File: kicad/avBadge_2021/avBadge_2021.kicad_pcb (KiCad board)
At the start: 2 copper layers, 115 x 75 mm, 37 parts, among them J1 AVR-ISP-6, Q1 2N3904, SW1 SW_Push_Dual, SW2 SW_SPDT, U1 ATtiny84A-SSU

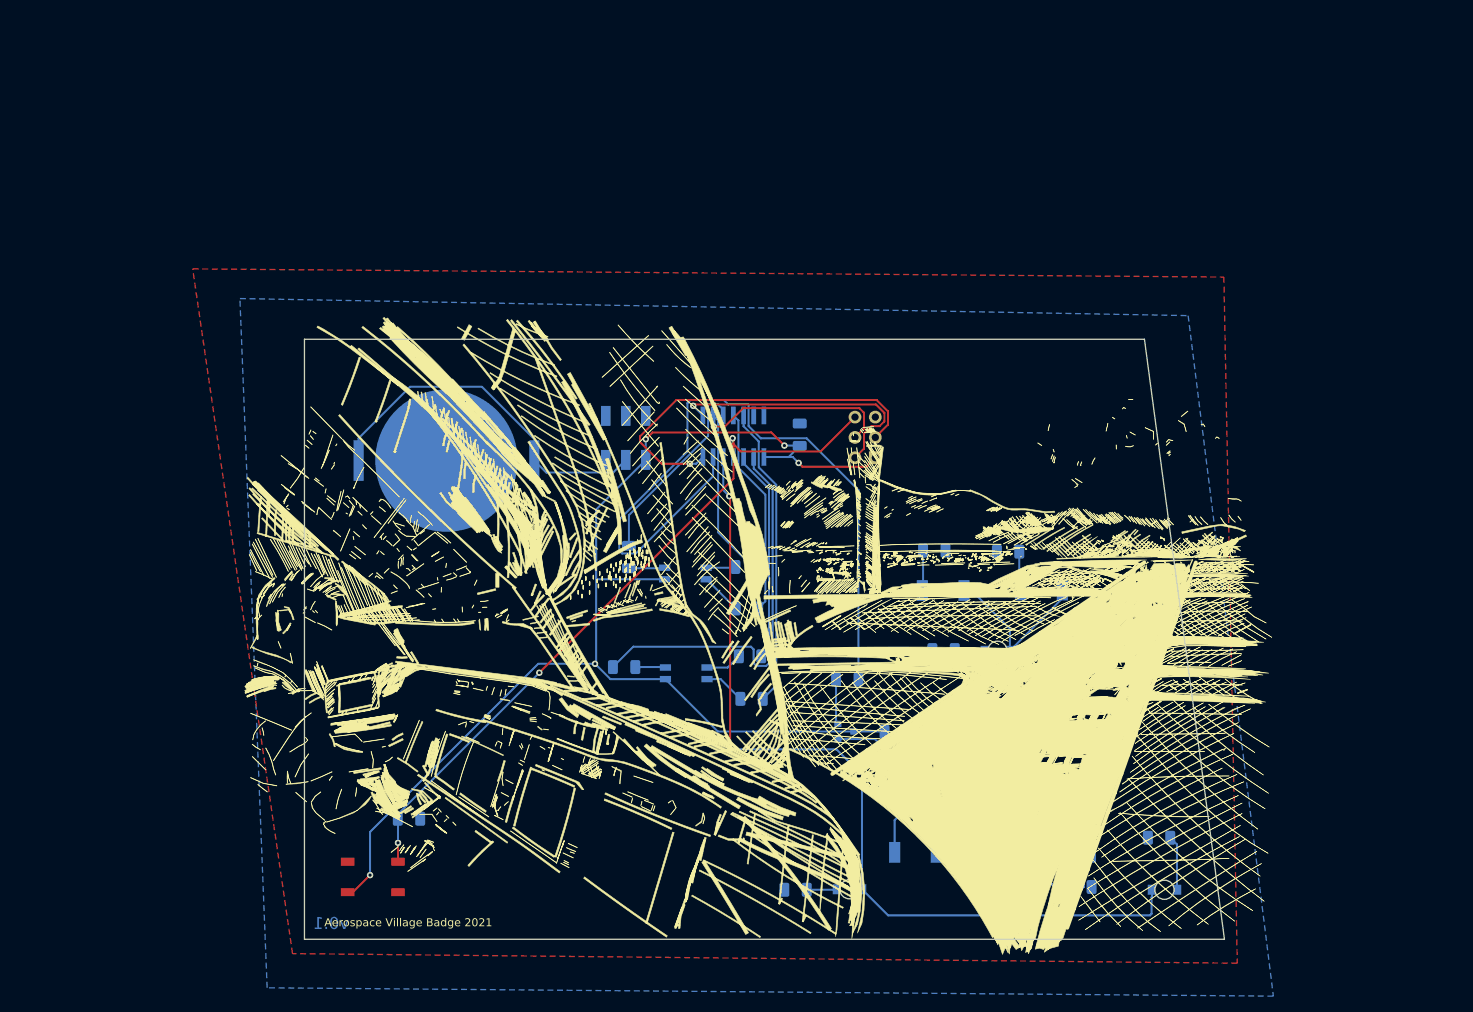
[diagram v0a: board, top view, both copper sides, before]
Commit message: v0.2 gerber builtout and sent for fabrication.
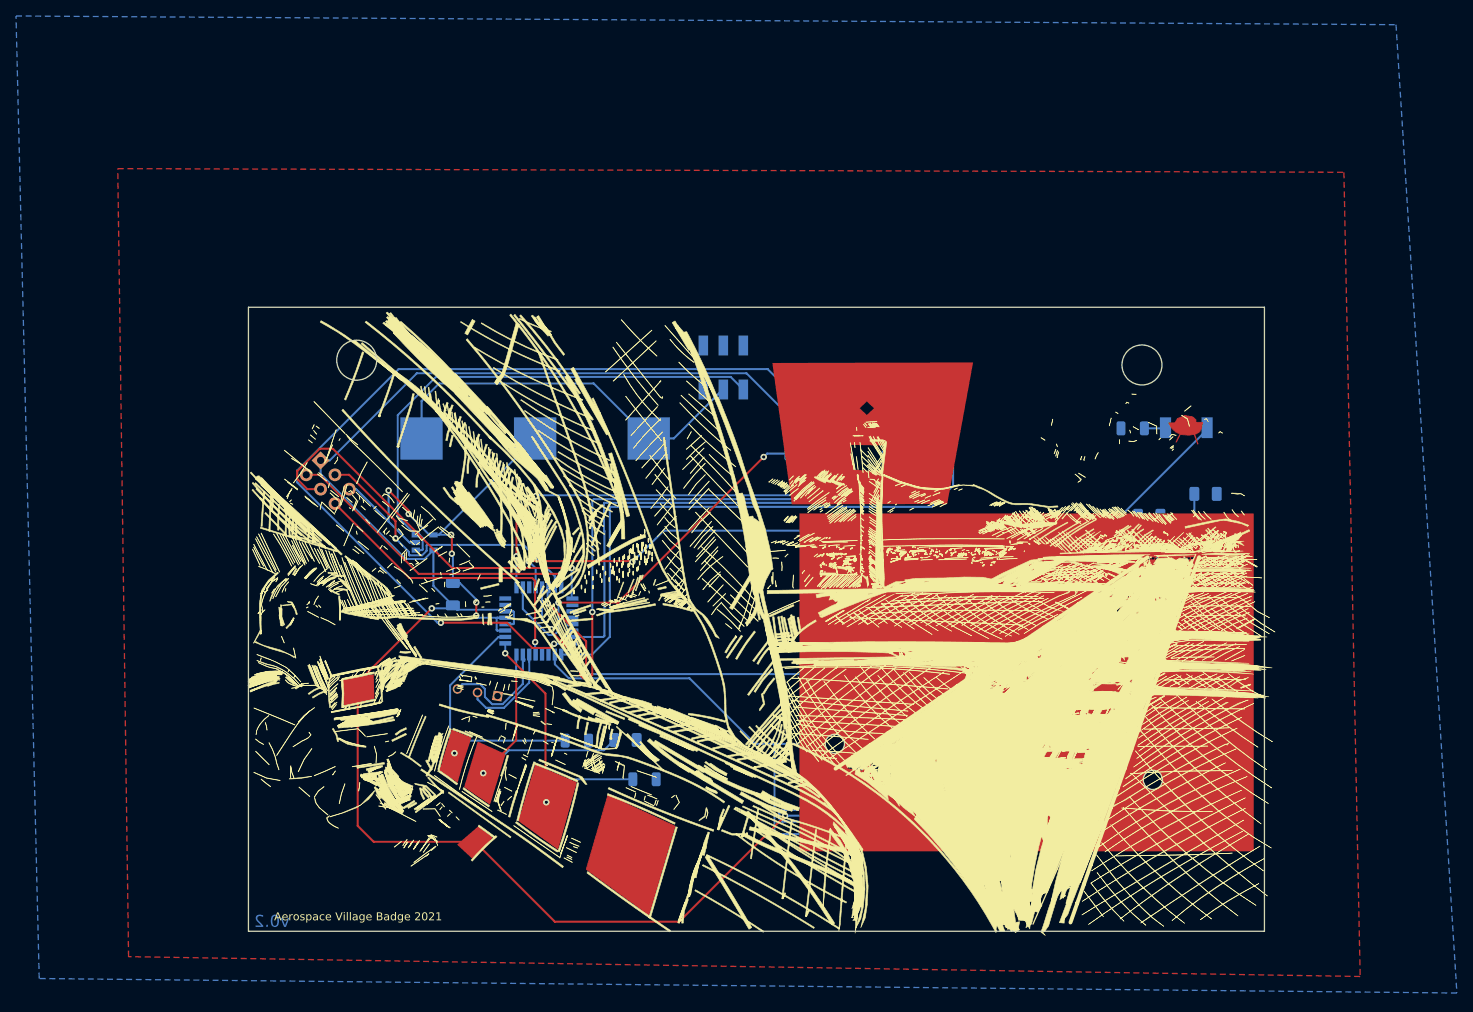
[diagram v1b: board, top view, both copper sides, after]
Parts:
- removed the D5 at (171.4, 134.1)
- removed the SW1 at (103.5, 137.2)
- removed svg2mod: G***, aerospace_badge:test
- added D12: LED, sunled:XZMYK45WT-9, B.Cu at (185.3, 117.4)
- added D4: LED, sunled:XZDGK45WT-9, B.Cu at (205.2, 81.1)
- added P1: SerialConnector, aerospace_badge:serialConnector, B.Cu at (116.6, 114.2)
- added R11: 330, Resistors_SMD:R_1206_3216Metric, B.Cu at (198.5, 81.1)
- added R12: 10K, Resistors_SMD:R_1206_3216Metric, B.Cu at (137.5, 125.0)
- added R7: 10K, Resistors_SMD:R_1206_3216Metric, B.Cu at (129.1, 120.2)
- added S1: OpenConnections, aerospace_badge:artboard, F.Cu at (150.5, 104.7)
- added VR1: TLV702, TO_SOT_Packages_SMD:SOT-23-5, B.Cu at (110.0, 95.4)
- BT1: footprint Battery:BatteryHolder_Keystone_3034_1x20mm -> aerospace_badge:BHX2-2032
- D1, D2: value APFA3010 -> SunLED_RGB_ReverseMount
- D10, D11: footprint aerospace_badge:led_in-s124ar -> sunled:XZMYK45WT-9
- D6: footprint sunled:XZDGK45WT-9 -> sunled:XZM2CRK45WT-9
- D8: footprint sunled:XZM2CRK45WT-9 -> sunled:XZDGK45WT-9
- D9: footprint aerospace_badge:led_in-s124ar -> sunled:XZDGK45WT-9
- J1: moved to F.Cu
- U1: value ATtiny84A-SSU -> ATmega8-16AU; footprint aerospace_badge:attiny84 -> digikey-footprints:TQFP-32_7x7mm
- moved J1 68.6 mm to (95.2, 86.9), turned to 45 degrees
- moved C1 47.7 mm to (113.6, 101.9)
- moved D1 40.1 mm to (165.4, 78.7)
- moved R2 35.1 mm to (172.6, 87.3)
- moved R4 34.6 mm to (157.0, 84.3)
- moved U1 33.5 mm to (124.3, 105.2), turned to 0 degrees
- moved R6 33.4 mm to (172.6, 84.3)
- moved R1 32.2 mm to (172.5, 80.4)
- moved R5 30.4 mm to (172.2, 77.4)
- moved R3 29.3 mm to (157.6, 77.9), turned to 0 degrees
- moved D7 29.1 mm to (188.9, 126.8)
- moved R9 28.8 mm to (135.1, 120.1)
- moved D11 28.4 mm to (197.3, 103.5), turned to 180 degrees
- moved D9 27.6 mm to (206.4, 96.8), turned to 270 degrees
- moved R19 27.3 mm to (201.6, 107.6), turned to 0 degrees
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- renumbered D4 to D5, R2 to R1, R8 to R10, R10 to R13, R11 to R14, R12 to R15, R13 to R16, R14 to R17, R15 to R18, R16 to R19, R1 to R2, R17 to R20, R4 to R3, R3 to R4, R6 to R5, R5 to R6, R7 to R8, SW2 to SW1
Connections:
- R1 pad 1: Net-(R2-Pad1) -> Net-(R1-Pad1)
- R1 pad 2: Net-(D2-Pad1) -> Net-(D1-Pad1)
- R13 pad 2: Net-(R10-Pad2) -> Net-(R13-Pad2)
- R14 pad 1: Net-(D5-Pad1) (its old number) -> Net-(D6-Pad1)
- R15 pad 1: Net-(D6-Pad1) -> Net-(D7-Pad1)
- R16 pad 1: Net-(D7-Pad1) -> Net-(D8-Pad1)
- R17 pad 1: Net-(D8-Pad1) -> Net-(D9-Pad1)
- R18 pad 1: Net-(D9-Pad1) -> Net-(D10-Pad1)
- R19 pad 1: Net-(D10-Pad1) -> Net-(D11-Pad1)
- R2 pad 1: Net-(R1-Pad1) -> Net-(R2-Pad1)
- R2 pad 2: Net-(D1-Pad1) -> Net-(D2-Pad1)
- R20 pad 1: Net-(D11-Pad1) -> Net-(D12-Pad1)
- R3 pad 1: Net-(R4-Pad1) -> Net-(R3-Pad1)
- R3 pad 2: Net-(D2-Pad3) -> Net-(D1-Pad3)
- R4 pad 1: Net-(R3-Pad1) -> Net-(R4-Pad1)
- R4 pad 2: Net-(D1-Pad3) -> Net-(D2-Pad3)
- R5 pad 1: Net-(J1-Pad3) -> Net-(R5-Pad1)
- R5 pad 2: Net-(D2-Pad4) -> Net-(D1-Pad4)
- R6 pad 1: Net-(R5-Pad1) -> Net-(R6-Pad1)
- R6 pad 2: Net-(D1-Pad4) -> Net-(D2-Pad4)
- R9 pad 2: Net-(J1-Pad5) -> Net-(R9-Pad2)
- SW1 pad 1: VCC -> Net-(SW1-Pad1)
- U1 pad 1: VCC -> Net-(R12-Pad2)
- U1 pad 11: Net-(R2-Pad1) -> Net-(U1-Pad11)
- U1 pad 12: Net-(R1-Pad1) -> Net-(D4-Pad2)
- U1 pad 13: Net-(U1-Pad13) -> Net-(R6-Pad1)
- U1 pad 14: GND -> Net-(R13-Pad2)
- U1 pad 2: Net-(R3-Pad1) -> Net-(R7-Pad2)
- U1 pad 3: Net-(R5-Pad1) -> GND
- U1 pad 4: Net-(J1-Pad5) -> VCC
- U1 pad 5: Net-(D3-Pad2) -> GND
- U1 pad 6: Net-(R10-Pad2) -> VCC
- U1 pad 7: Net-(J1-Pad4) -> Net-(U1-Pad7)
- U1 pad 8: Net-(J1-Pad1) -> Net-(U1-Pad8)
- U1 pad 9: Net-(J1-Pad3) -> Net-(R2-Pad1)
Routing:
- net GND: track 0.00 -> 128.6 mm, vias 0 -> 6
- net Net-(D4-Pad2): track 0.00 -> 95.6 mm, vias 0 -> 2
- net Net-(R10-Pad2): track 91.8 -> 0.00 mm
- net VCC: track 166.1 -> 257.8 mm, vias 5 -> 2
- net Net-(R6-Pad1): track 0.00 -> 85.8 mm, vias 0 -> 2
- net Net-(SW1-Pad1): track 0.00 -> 65.1 mm
- net Net-(R3-Pad1): track 50.4 -> 114.3 mm, vias 0 -> 3
- net Net-(R13-Pad2): track 0.00 -> 53.7 mm, vias 0 -> 2
- net Net-(R5-Pad1): track 26.6 -> 79.2 mm
- net Net-(J1-Pad5): track 90.1 -> 38.3 mm, vias 3 -> 1
- net Net-(R2-Pad1): track 26.2 -> 63.4 mm, vias 0 -> 2
- net Net-(R1-Pad1): track 38.4 -> 73.3 mm
- net Net-(R9-Pad2): track 0.00 -> 34.6 mm, vias 0 -> 2
- net Net-(R12-Pad2): track 0.00 -> 34.2 mm, vias 0 -> 2
- net Net-(R7-Pad2): track 0.00 -> 32.6 mm, vias 0 -> 1
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- added copper zone on F.Cu, net GND
- removed copper zone on F.Cu, net VCC
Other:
- board size 115 x 75 mm -> 127 x 78 mm
- rule pad_to_mask_clearance: 0.05 -> 0
- board text added: "v0.2"
- board text removed: "v0.1"
